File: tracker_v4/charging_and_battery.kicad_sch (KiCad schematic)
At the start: 20 parts, among them J1 USB_C_Receptacle_USB2.0_16P, Q1 DMG9926UDM-7, U3 DW01A, U5 TP4056-42-ESOP8

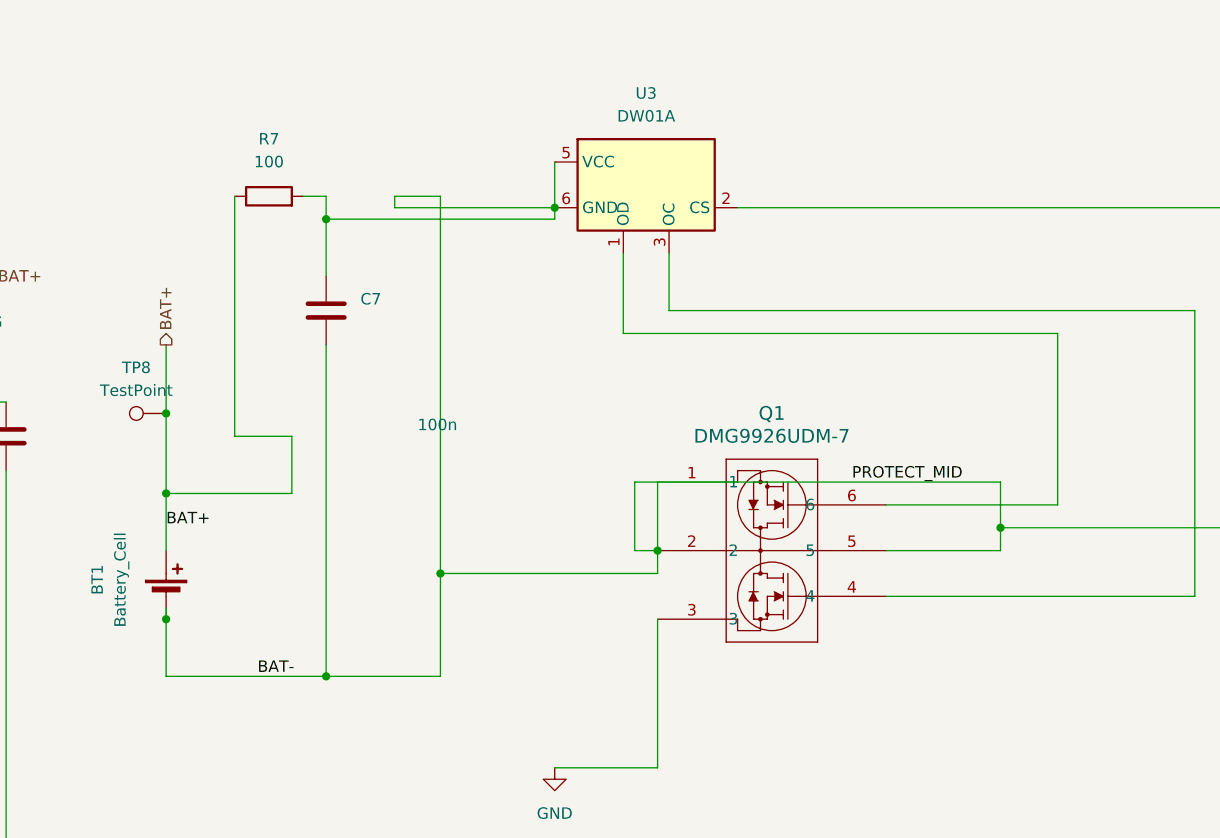
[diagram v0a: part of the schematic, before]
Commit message: m
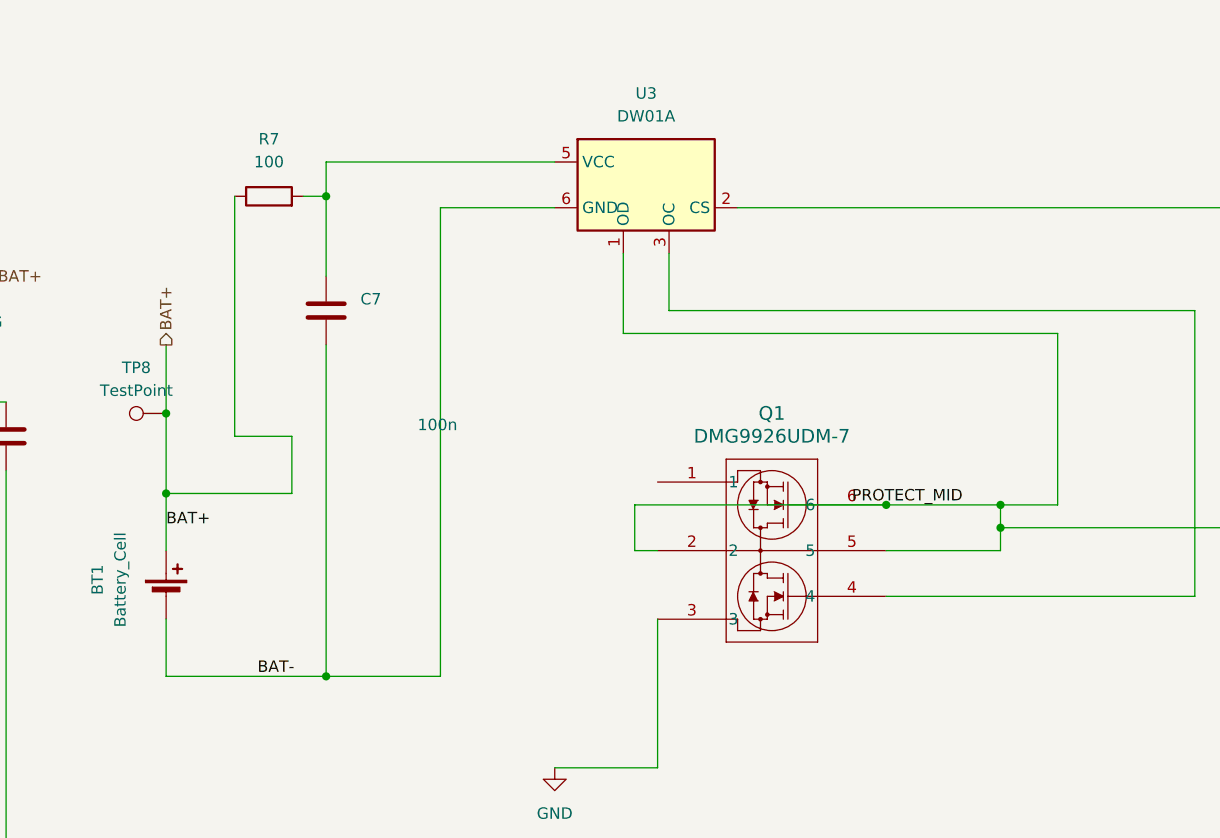
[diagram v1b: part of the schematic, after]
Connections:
- net BAT-: no longer C7.1, Q1.1, Q1.2, Q1.5, R7.2, R9.2, U3.5 (VCC)
- net PROTECT_MID: now reaches Q1.6, U3.1 (OD)
- net PROTECT_MID: now also Q1.2, Q1.5, R9.2
- new net: C7.1, R7.2, U3.5 (VCC)
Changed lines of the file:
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@@
+	)
+	(junction
+		(at 209.55 115.57)
+		(diameter 0)
+		(color 0 0 0 0)
 	)
 	(junction
@@
 	)
 	(junction
-		(at 184.15 120.65)
-		(diameter 0)
-		(color 0 0 0 0)
-	)
-	(junction
-		(at 129.54 128.27)
-		(diameter 0)
-		(color 0 0 0 0)
-	)
-	(junction
 		(at 222.25 118.11)
 		(diameter 0)
@@
 	)
 	(junction
+		(at 147.32 81.28)
+		(diameter 0)
+		(color 0 0 0 0)
+	)
+	(junction
 		(at 31.75 163.83)
 		(diameter 0)
@@
 	)
 	(junction
-		(at 172.72 82.55)
-		(diameter 0)
-		(color 0 0 0 0)
-	)
-	(junction
 		(at 67.31 78.74)
 		(diameter 0)
@@
 	)
 	(junction
-		(at 160.02 123.19)
-		(diameter 0)
-		(color 0 0 0 0)
-	)
-	(junction
 		(at 129.54 114.3)
 		(diameter 0)
@@
 	)
 	(junction
-		(at 147.32 83.82)
-		(diameter 0)
-		(color 0 0 0 0)
-	)
-	(junction
 		(at 101.6 90.17)
+		(diameter 0)
+		(color 0 0 0 0)
+	)
+	(junction
+		(at 222.25 115.57)
 		(diameter 0)
 		(color 0 0 0 0)
@@
 	(wire
 		(pts
-			(xy 160.02 134.62) (xy 160.02 123.19)
-		)
-		(stroke
-			(width 0)
-			(type default)
-		)
-	)
-	(wire
-		(pts
-			(xy 172.72 82.55) (xy 172.72 77.47)
-		)
-		(stroke
-			(width 0)
-			(type default)
-		)
-	)
-	(wire
-		(pts
-			(xy 160.02 81.28) (xy 160.02 123.19)
+			(xy 147.32 81.28) (xy 147.32 90.17)
 		)
 		(stroke
@@
 	(wire
 		(pts
-			(xy 129.54 134.62) (xy 129.54 128.27)
-		)
-		(stroke
-			(width 0)
-			(type default)
-		)
-	)
-	(wire
-		(pts
 			(xy 64.77 106.68) (xy 64.77 113.03)
 		)
@@
 	(wire
 		(pts
+			(xy 147.32 77.47) (xy 147.32 81.28)
+		)
+		(stroke
+			(width 0)
+			(type default)
+		)
+	)
+	(wire
+		(pts
 			(xy 55.88 134.62) (xy 55.88 163.83)
 		)
@@
 	(wire
 		(pts
-			(xy 184.15 123.19) (xy 184.15 120.65)
-		)
-		(stroke
-			(width 0)
-			(type default)
-		)
-	)
-	(wire
-		(pts
 			(xy 52.07 55.88) (xy 52.07 54.61)
 		)
@@
 	(wire
 		(pts
-			(xy 181.61 120.65) (xy 181.61 113.03)
-		)
-		(stroke
-			(width 0)
-			(type default)
-		)
-	)
-	(wire
-		(pts
-			(xy 129.54 127) (xy 129.54 128.27)
+			(xy 181.61 120.65) (xy 181.61 115.57)
 		)
 		(stroke
@@
 	(wire
 		(pts
-			(xy 181.61 113.03) (xy 222.25 113.03)
+			(xy 181.61 115.57) (xy 209.55 115.57)
 		)
 		(stroke
@@
 	(wire
 		(pts
-			(xy 147.32 83.82) (xy 172.72 83.82)
-		)
-		(stroke
-			(width 0)
-			(type default)
-		)
-	)
-	(wire
-		(pts
 			(xy 55.88 96.52) (xy 55.88 127)
 		)
@@
 	(wire
 		(pts
+			(xy 172.72 77.47) (xy 147.32 77.47)
+		)
+		(stroke
+			(width 0)
+			(type default)
+		)
+	)
+	(wire
+		(pts
 			(xy 129.54 134.62) (xy 147.32 134.62)
 		)
@@
 	(wire
 		(pts
-			(xy 160.02 81.28) (xy 154.94 81.28)
-		)
-		(stroke
-			(width 0)
-			(type default)
-		)
-	)
-	(wire
-		(pts
 			(xy 76.2 113.03) (xy 78.74 113.03)
 		)
@@
 	(wire
 		(pts
-			(xy 154.94 81.28) (xy 154.94 82.55)
-		)
-		(stroke
-			(width 0)
-			(type default)
-		)
-	)
-	(wire
-		(pts
 			(xy 50.8 85.09) (xy 50.8 146.05)
 		)
@@
 	(wire
 		(pts
-			(xy 172.72 83.82) (xy 172.72 82.55)
+			(xy 160.02 82.55) (xy 172.72 82.55)
+		)
+		(stroke
+			(width 0)
+			(type default)
+		)
+	)
+	(wire
+		(pts
+			(xy 209.55 115.57) (xy 222.25 115.57)
 		)
 		(stroke
@@
 	(wire
 		(pts
-			(xy 184.15 120.65) (xy 184.15 113.03)
-		)
-		(stroke
-			(width 0)
-			(type default)
-		)
-	)
-	(wire
-		(pts
-			(xy 154.94 82.55) (xy 172.72 82.55)
-		)
-		(stroke
-			(width 0)
-			(type default)
-		)
-	)
-	(wire
-		(pts
 			(xy 172.72 144.78) (xy 184.15 144.78)
 		)
@@
 	(wire
 		(pts
+			(xy 129.54 128.27) (xy 129.54 134.62)
+		)
+		(stroke
+			(width 0)
+			(type default)
+		)
+	)
+	(wire
+		(pts
 			(xy 129.54 97.79) (xy 129.54 105.41)
 		)
@@
 	(wire
 		(pts
-			(xy 147.32 83.82) (xy 147.32 90.17)
-		)
-		(stroke
-			(width 0)
-			(type default)
-		)
-	)
-	(wire
-		(pts
 			(xy 67.31 78.74) (xy 78.74 78.74)
 		)
@@
 	(wire
 		(pts
-			(xy 222.25 113.03) (xy 222.25 118.11)
-		)
-		(stroke
-			(width 0)
-			(type default)
-		)
-	)
-	(wire
-		(pts
-			(xy 209.55 115.57) (xy 228.6 115.57)
+			(xy 222.25 115.57) (xy 222.25 118.11)
 		)
 		(stroke
@@
 	(wire
 		(pts
-			(xy 147.32 81.28) (xy 147.32 83.82)
-		)
-		(stroke
-			(width 0)
-			(type default)
-		)
-	)
-	(wire
-		(pts
 			(xy 228.6 96.52) (xy 180.34 96.52)
 		)
@@
 	(wire
 		(pts
+			(xy 222.25 115.57) (xy 228.6 115.57)
+		)
+		(stroke
+			(width 0)
+			(type default)
+		)
+	)
+	(wire
+		(pts
 			(xy 76.2 107.95) (xy 76.2 113.03)
 		)
@@
 	(wire
 		(pts
-			(xy 160.02 123.19) (xy 184.15 123.19)
-		)
-		(stroke
-			(width 0)
-			(type default)
-		)
-	)
-	(wire
-		(pts
 			(xy 91.44 129.54) (xy 91.44 134.62)
 		)
@@
 	(wire
 		(pts
+			(xy 160.02 82.55) (xy 160.02 134.62)
+		)
+		(stroke
+			(width 0)
+			(type default)
+		)
+	)
+	(wire
+		(pts
 			(xy 59.69 34.29) (xy 59.69 30.48)
 		)
@@
 	)
 	(label "PROTECT_MID"
-		(at 205.74 113.03 0)
+		(at 205.74 115.57 0)
 		(effects
 			(font
